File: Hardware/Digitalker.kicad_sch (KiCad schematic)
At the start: 4 parts, among them U2 SN74LVC245APW, U3 SN74LVC245APW, U4 SN74LVC8T245, X1 ICSockets-40P

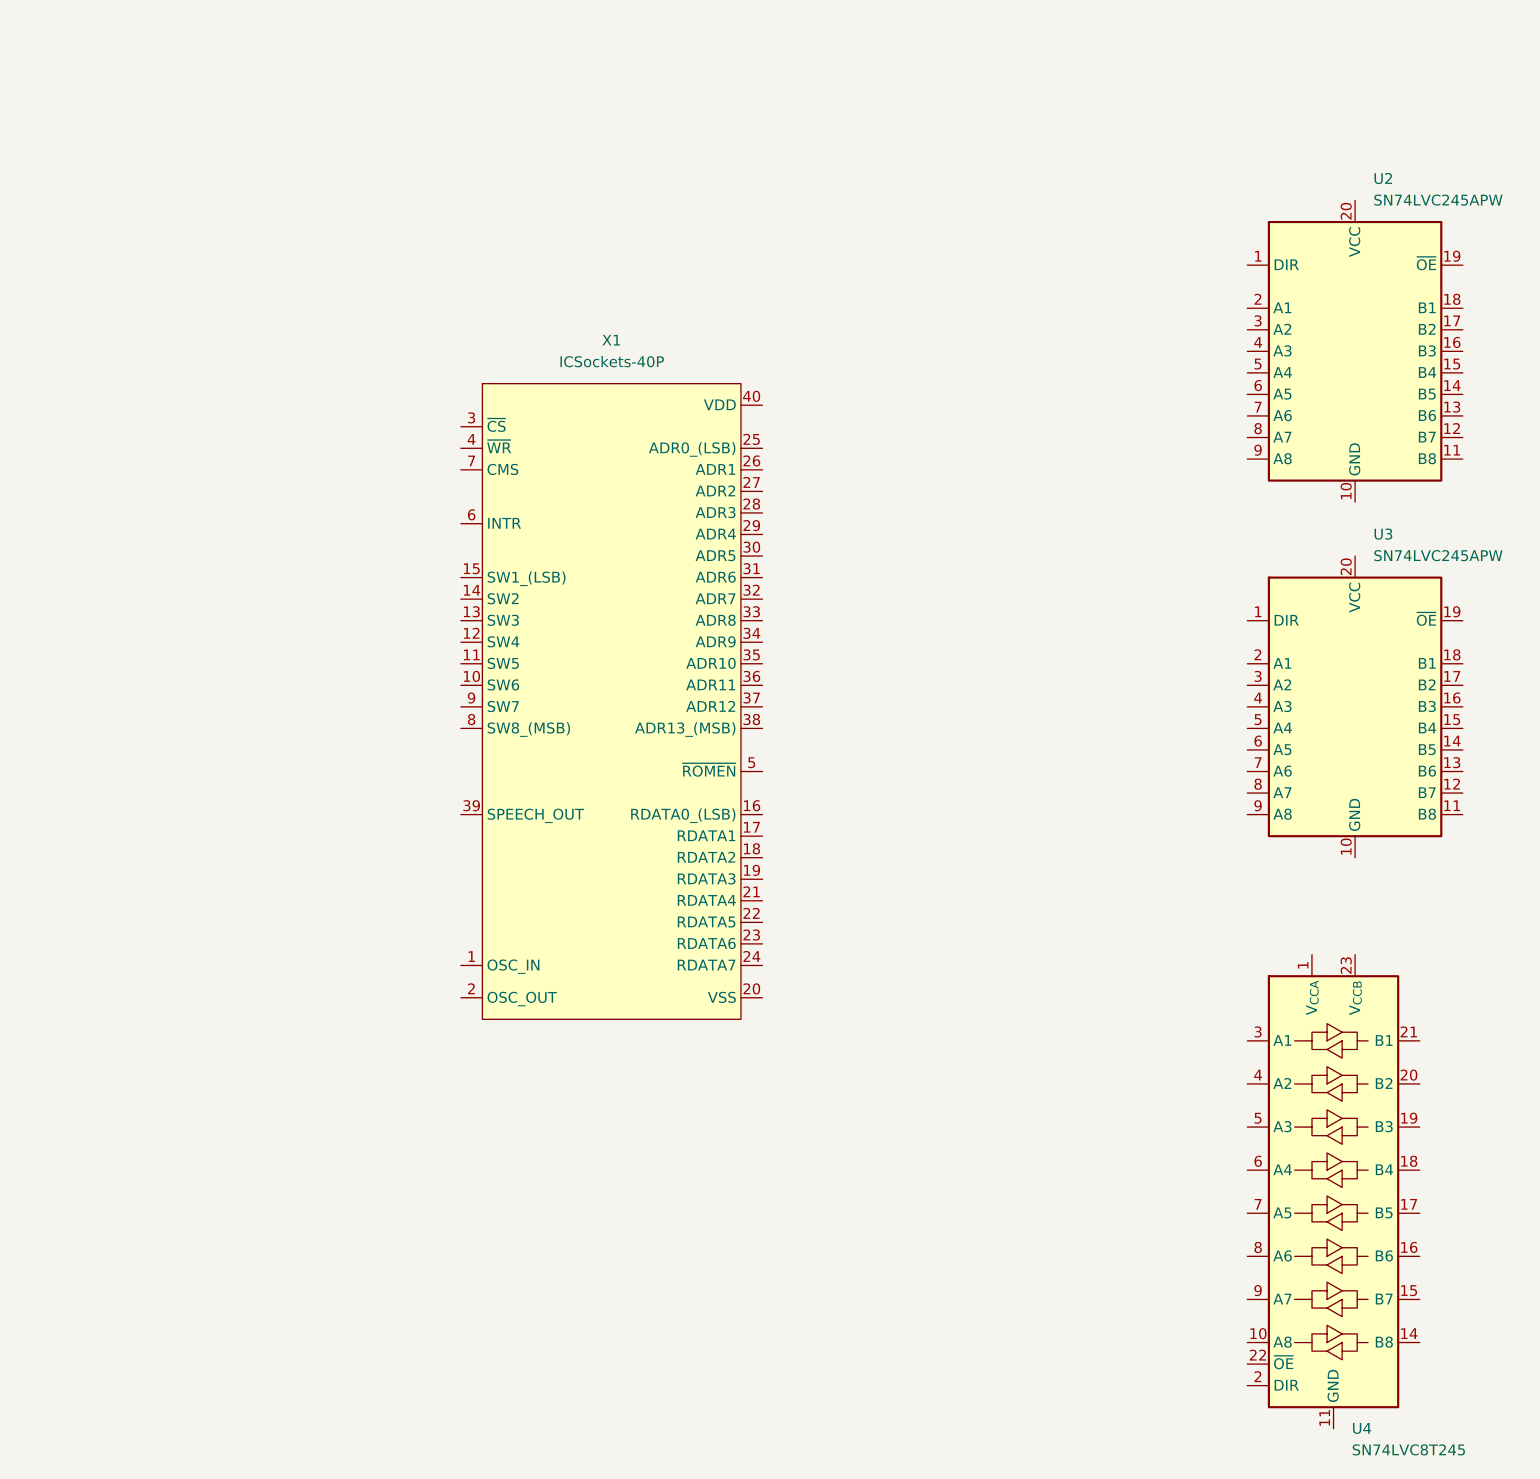
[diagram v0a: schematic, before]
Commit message: digitalker work
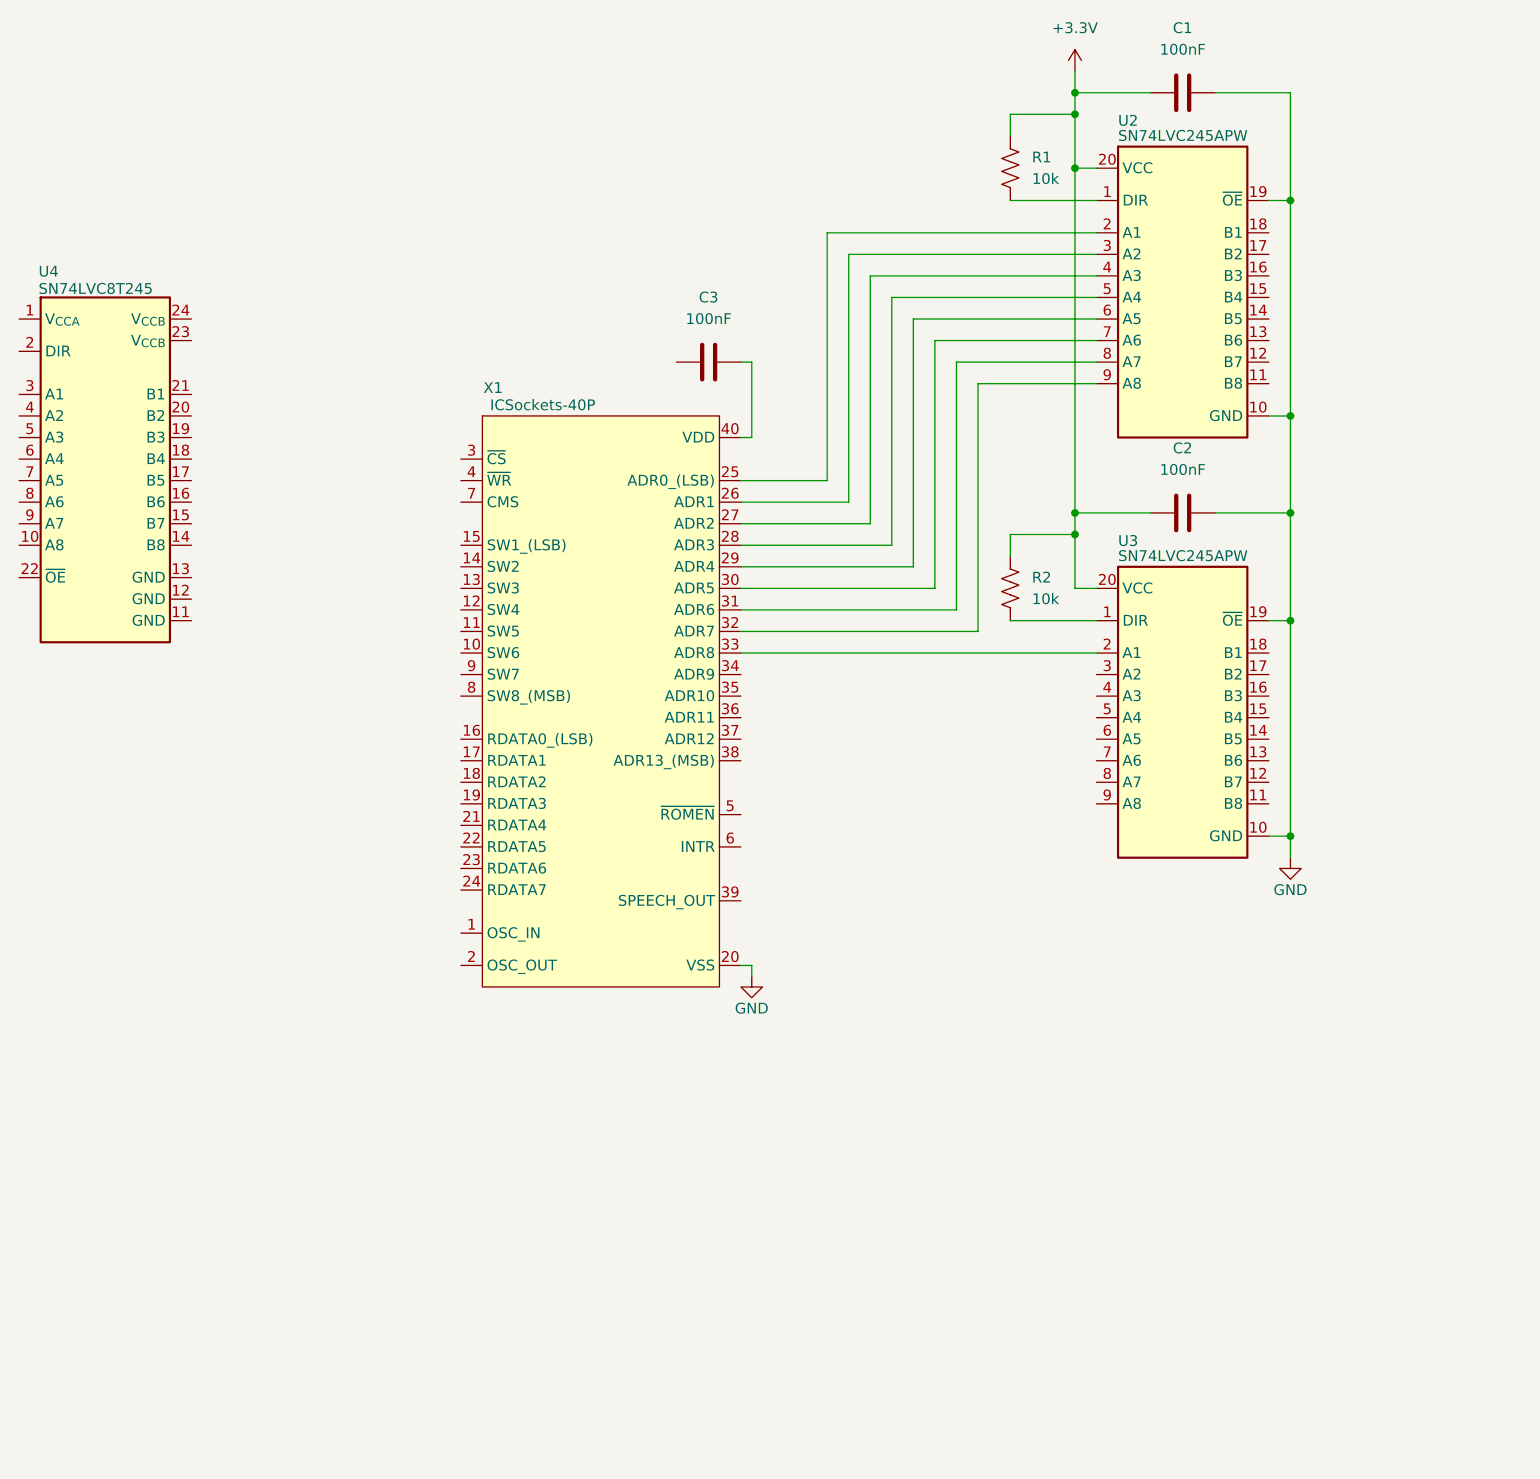
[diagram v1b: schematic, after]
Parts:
- added C1, C2, C3: 100nF, symbol Device:C
- added R1, R2: 10k, symbol Device:R_US
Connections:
- net at U3.1 (DIR): now also R2.1
- net GND: now reaches U3.10 (GND)
- net GND: now also U2.10 (GND), U2.19 (~{OE}), U3.19 (~{OE}), X1.20 (VSS), C1.1, C2.1
- net at U3.2 (A1): now also X1.33 (ADR8)
- net +3.3V: now reaches U3.20 (VCC)
- net +3.3V: now also U2.20 (VCC), C1.2, C2.2, R1.2, R2.2
- net at U2.1 (DIR): now also R1.1
- net at U2.2 (A1): now also X1.25 (ADR0_(LSB))
- net at U2.3 (A2): now also X1.26 (ADR1)
- net at U2.4 (A3): now also X1.27 (ADR2)
- net at U2.5 (A4): now also X1.28 (ADR3)
- net at U2.6 (A5): now also X1.29 (ADR4)
- net at U2.7 (A6): now also X1.30 (ADR5)
- net at U2.8 (A7): now also X1.31 (ADR6)
- net at U2.9 (A8): now also X1.32 (ADR7)
- net at U4.23 (V_{CCB}): no longer U4.24 (V_{CCB})
- net at X1.40 (VDD): now also C3.1
- now unconnected: U4.11 (GND), U4.12 (GND), U4.13 (GND)
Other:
- moved on the sheet: U2, X1
